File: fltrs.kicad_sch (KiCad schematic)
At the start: 25 parts, among them U4 MCP6002, U5 MCP6002, U6 MCP4551

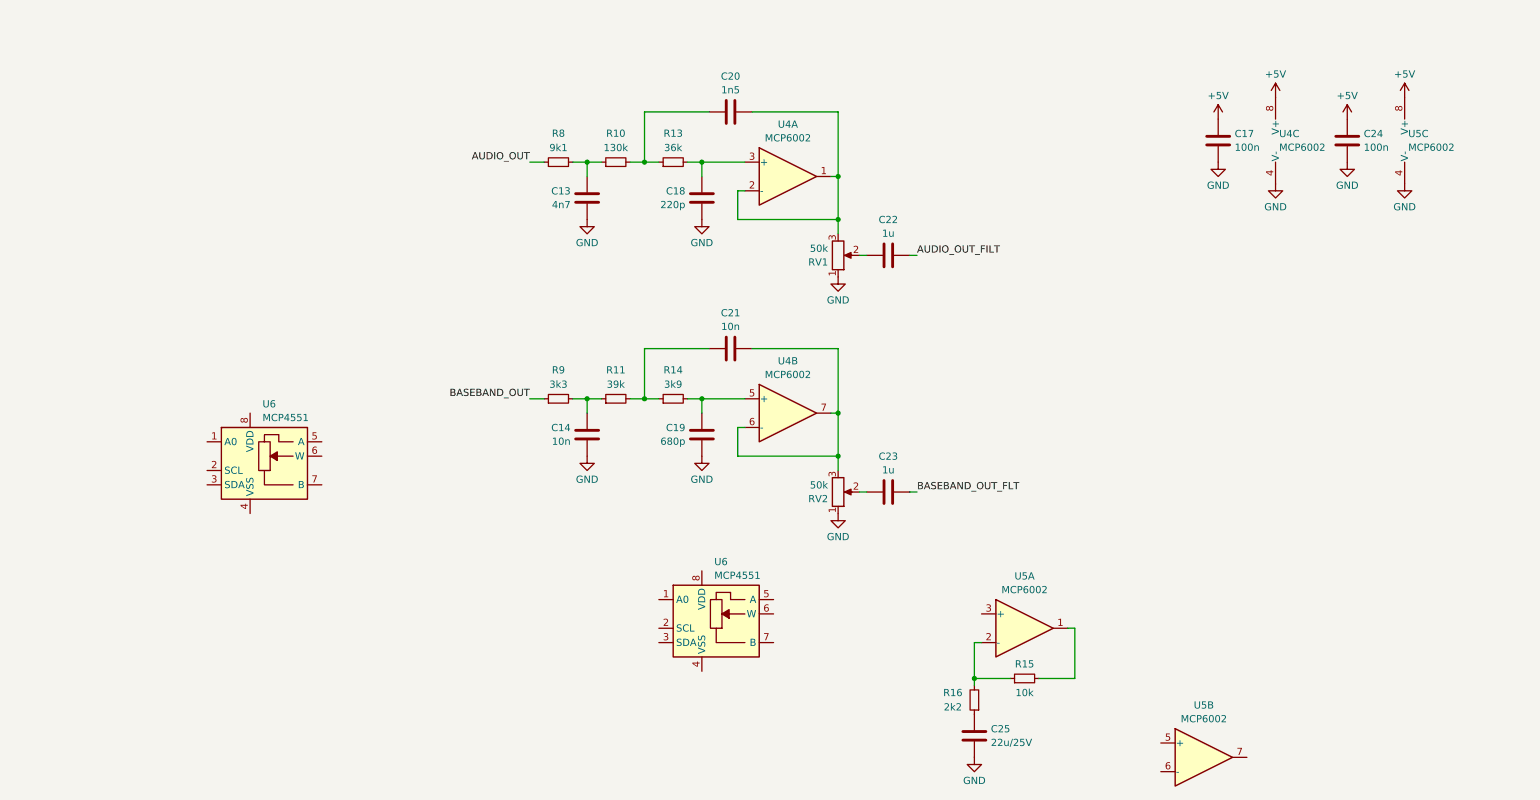
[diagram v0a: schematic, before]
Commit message: WIP filters
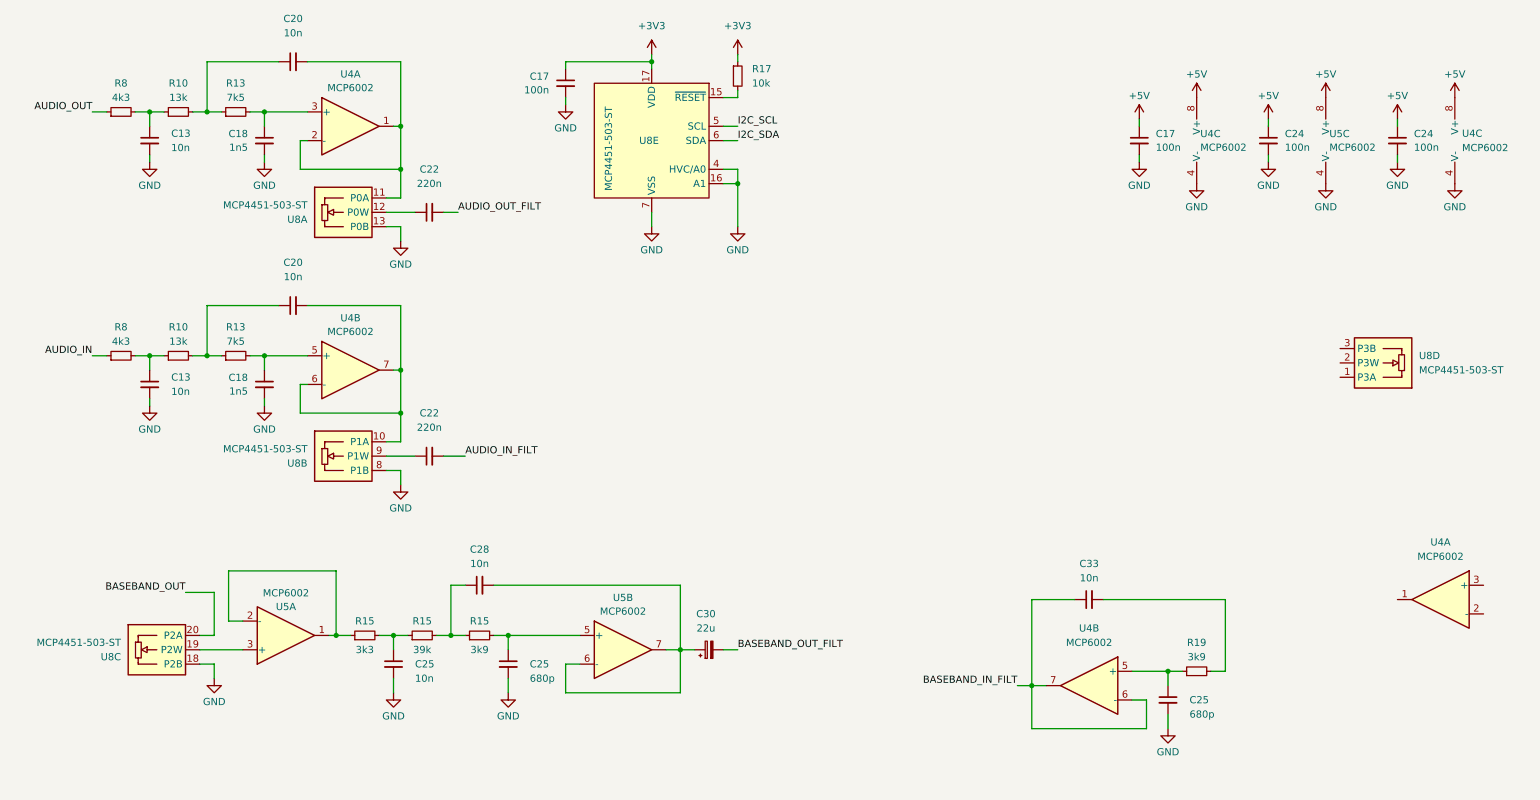
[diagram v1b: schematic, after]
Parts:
- removed C14, C21: 10n, Capacitor_SMD:C_0603_1608Metric, symbol Device:C
- removed C19: 680p, Capacitor_SMD:C_0603_1608Metric, symbol Device:C
- removed C23: 1u, Capacitor_SMD:C_0603_1608Metric, symbol Device:C
- removed R11: 39k, Resistor_SMD:R_0603_1608Metric, symbol Device:R_Small
- removed R14: 3k9, Resistor_SMD:R_0603_1608Metric, symbol Device:R_Small
- removed R16: 2k2, Resistor_SMD:R_0603_1608Metric, symbol Device:R_Small
- removed R9: 3k3, Resistor_SMD:R_0603_1608Metric, symbol Device:R_Small
- removed RV1: 50k, symbol Device:R_Potentiometer
- removed RV2: 50k, Potentiometer_SMD:Potentiometer_Bourns_3224J_Horizontal, symbol Device:R_Potentiometer
- removed U6 (x2): MCP4551, Package_SO:MSOP-8_3x3mm_P0.65mm, symbol micro17:MCP4551
- added C13, C20: 10n, Capacitor_SMD:C_0603_1608Metric, symbol Device:C_Small
- added C17, C24: 100n, Capacitor_SMD:C_0603_1608Metric, symbol Device:C_Small
- added C18: 1n5, Capacitor_SMD:C_0603_1608Metric, symbol Device:C_Small
- added C22: 220n, Capacitor_SMD:C_0603_1608Metric, symbol Device:C_Small
- added C25 (x2): 680p, Capacitor_SMD:C_0805_2012Metric, symbol Device:C_Small
- added C28, C33: 10n, symbol Device:C_Small
- added C30: 22u, symbol Device:C_Polarized_Small
- added R10: 13k, Resistor_SMD:R_0603_1608Metric, symbol Device:R_Small
- added R13: 7k5, Resistor_SMD:R_0603_1608Metric, symbol Device:R_Small
- added R15: 39k, Resistor_SMD:R_0603_1608Metric, symbol Device:R_Small
- added R15: 3k9, Resistor_SMD:R_0603_1608Metric, symbol Device:R_Small
- added R17: 10k, symbol Device:R_Small
- added R19: 3k9, symbol Device:R_Small
- added R8: 4k3, Resistor_SMD:R_0603_1608Metric, symbol Device:R_Small
- added U4: MCP6002, Package_DFN_QFN:DFN-8-1EP_3x2mm_P0.5mm_EP1.75x1.45mm, symbol Amplifier_Operational:MCP6002-xMC
- added U8: MCP4451-503-ST, Package_SO:TSSOP-20_4.4x6.5mm_P0.65mm, symbol Potentiometer_Digital:MCP4451-xxxx-ST
- C13: value 4n7 -> 10n; symbol Device:C -> Device:C_Small
- C17, C24: symbol Device:C -> Device:C_Small
- C18: value 220p -> 1n5; symbol Device:C -> Device:C_Small
- C20: value 1n5 -> 10n; symbol Device:C -> Device:C_Small
- C22: value 1u -> 220n; symbol Device:C -> Device:C_Small
- C25: value 22u/25V -> 10n; symbol Device:C -> Device:C_Small
- R10: value 130k -> 13k
- R13: value 36k -> 7k5
- R15: value 10k -> 3k3
- R8: value 9k1 -> 4k3
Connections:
- net +5V: now also C24.1, U4.8 (V+)
- net BASEBAND_OUT: now also U8.20 (P2A)
- net GND: now also C13.2, C17.2, C18.2, C24.2, C25.2, C25.2, U4.4 (V-), U4.9 (V-), U8.13 (P0B), U8.16 (A1), U8.18 (P2B), U8.4 (HVC/A0), U8.7 (VSS), U8.8 (P1B)
- net at U4.5 (+): now also C18.1, R13.2
- net at U4.6 (-), U4.7: now also C20.2, U8.10 (P1A)
- net at U5.1: now also R15.1, U5.2 (-); no longer R15.2
- net at U5.3 (+): now also U8.19 (P2W)
- net at C22.1: now also U8.12 (P0W)
- net at C20.2, U4.1, U4.2 (-): now also U8.11 (P0A)
- net at U5.5 (+): now also C25.1, R15.2
- net at U5.6 (-): now also U5.7, C28.2, C30.1
- net at C25.1: now also R15.2, R15.1
- new net: C20.1, R10.2, R13.1
- new net: C28.1, R15.1, R15.2
- new net: C22.1, U8.9 (P1W)
- new net: R17.2, U8.15 (~{RESET})
- new net: C25.1, R19.1, U4.5 (+)
- new net: C33.2, R19.2
- new net: C13.1, R10.1, R8.2
- new net +3V3: C17.1, R17.1, U8.17 (VDD)
- new net AUDIO_IN: R8.1
- new net AUDIO_IN_FILT: C22.2
- new net BASEBAND_IN_FILT: C33.1, U4.6 (-), U4.7
- new net BASEBAND_OUT_FILT: C30.2
- new net I2C_SCL: U8.5 (SCL)
- new net I2C_SDA: U8.6 (SDA)
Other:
- moved on the sheet: C13, C17, C18, C20, C22, C24, C25, R10, R13, R15, R8, U4A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
